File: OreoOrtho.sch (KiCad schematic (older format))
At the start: 31 parts, among them SW1 MXSwitch, SW2 MXSwitch, SW3 MXSwitch, SW4 MXSwitch, U1 ATmega32U2-AU, U2 PRTR5V0U2X, Y1 16MHz

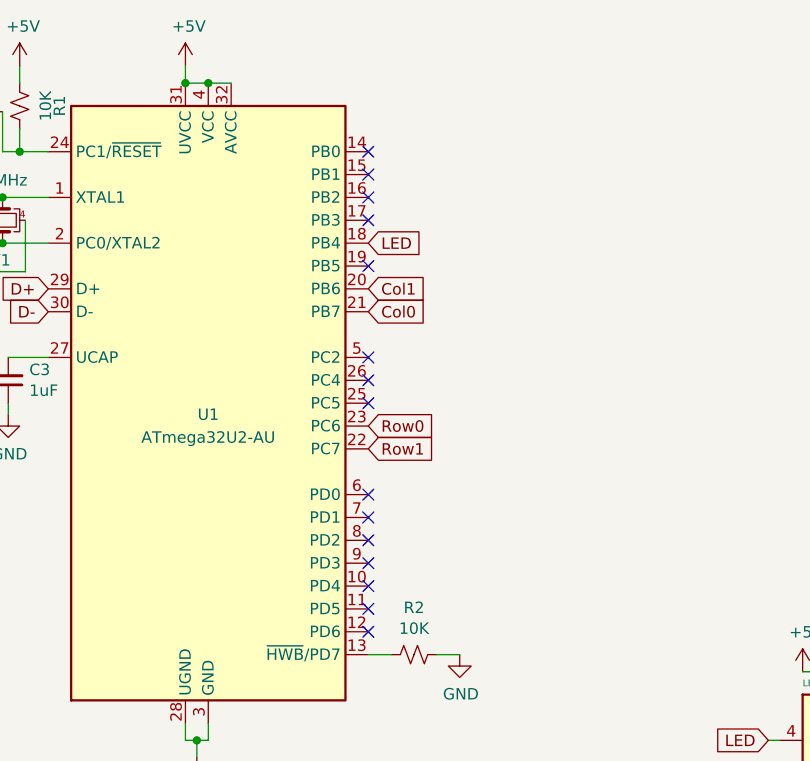
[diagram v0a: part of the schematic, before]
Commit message: reroute
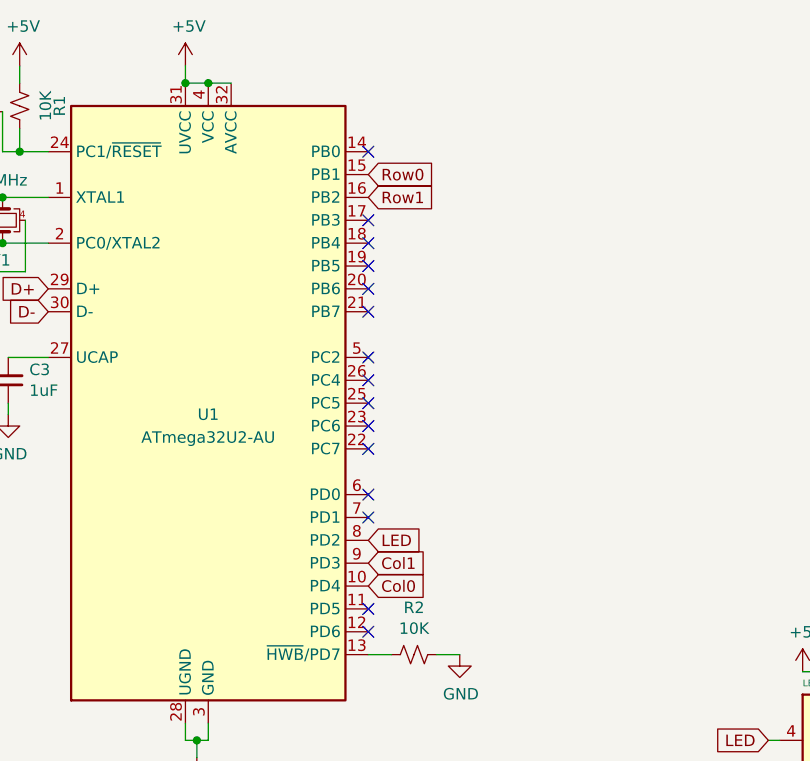
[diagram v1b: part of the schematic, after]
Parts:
- SW1, SW2, SW3, SW4: footprint kbd:CherryMX_1u -> kbd:CherryMX_Hotswap
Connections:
- net Col0: now also U1.10 (PD4); no longer U1.21 (PB7)
- net Col1: now also U1.9 (PD3); no longer U1.20 (PB6)
- net LED: now also U1.8 (PD2); no longer U1.18 (PB4)
- net Row0: now also U1.15 (PB1); no longer U1.23 (PC6)
- net Row1: now also U1.16 (PB2); no longer U1.22 (PC7)
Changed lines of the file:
@@
 Wire Wire Line
 	1925 4250 1925 4450
-Text GLabel 5825 2725 2    50   Input ~ 0
+Text GLabel 5825 1625 2    50   Input ~ 0
 Row1
-Text GLabel 5825 2025 2    50   Input ~ 0
+Text GLabel 5825 3225 2    50   Input ~ 0
 Col1
 $Comp
@@
 $EndComp
 NoConn ~ 5825 1425
-NoConn ~ 5825 1525
-NoConn ~ 5825 1625
+NoConn ~ 5825 2725
+NoConn ~ 5825 2625
 NoConn ~ 5825 2925
 NoConn ~ 5825 3025
-NoConn ~ 5825 3125
-NoConn ~ 5825 3225
-NoConn ~ 5825 3325
+NoConn ~ 5825 2025
+NoConn ~ 5825 1825
+NoConn ~ 5825 2125
 NoConn ~ 5825 3425
 NoConn ~ 5825 3525
@@
 F 0 "SW3" H 8250 1950 50  0000 L CNN
 F 1 "MXSwitch" H 8175 1875 39  0000 L CNN
-F 2 "kbd:CherryMX_1u" H 8325 1950 50  0001 C CNN
+F 2 "kbd:CherryMX_Hotswap" H 8325 1950 50  0001 C CNN
 F 3 "" H 8325 1950 50  0001 C CNN
 	1    8325 1950
@@
 F 0 "SW4" H 8950 1950 50  0000 L CNN
 F 1 "MXSwitch" H 8875 1875 39  0000 L CNN
-F 2 "kbd:CherryMX_1u" H 9025 1950 50  0001 C CNN
+F 2 "kbd:CherryMX_Hotswap" H 9025 1950 50  0001 C CNN
 F 3 "" H 9025 1950 50  0001 C CNN
 	1    9025 1950
@@
 F 0 "SW1" H 8250 1375 50  0000 L CNN
 F 1 "MXSwitch" H 8175 1300 39  0000 L CNN
-F 2 "kbd:CherryMX_1u" H 8325 1375 50  0001 C CNN
+F 2 "kbd:CherryMX_Hotswap" H 8325 1375 50  0001 C CNN
 F 3 "" H 8325 1375 50  0001 C CNN
 	1    8325 1375
@@
 	1    0    0    -1
 $EndComp
-Text GLabel 5825 2125 2    50   Input ~ 0
+Text GLabel 5825 3325 2    50   Input ~ 0
 Col0
-Text GLabel 5825 2625 2    50   Input ~ 0
+Text GLabel 5825 1525 2    50   Input ~ 0
 Row0
 NoConn ~ 5825 1725
-Text GLabel 5825 1825 2    50   Input ~ 0
+Text GLabel 5825 3125 2    50   Input ~ 0
 LED
 $Comp
@@
 F 0 "SW2" H 8950 1375 50  0000 L CNN
 F 1 "MXSwitch" H 8875 1300 39  0000 L CNN
-F 2 "kbd:CherryMX_1u" H 9025 1375 50  0001 C CNN
+F 2 "kbd:CherryMX_Hotswap" H 9025 1375 50  0001 C CNN
 F 3 "" H 9025 1375 50  0001 C CNN
 	1    9025 1375

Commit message: minor file changes
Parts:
- added C7: 0.1uF, Capacitor_SMD:C_0603_1608Metric, symbol Device:C_Small
- added G2: Oreo, doggy:bike, symbol oreo:LOGO
- SW1, SW2, SW3, SW4: footprint kbd:CherryMX_Hotswap -> doggy:CherryMX_Hotswap_clear
- U1: value ATmega32U2-AU -> ATmega32U4-AU; footprint Package_QFP:TQFP-32_7x7mm_P0.8mm -> Package_QFP:TQFP-44_10x10mm_P0.8mm; symbol MCU_Microchip_ATmega:ATmega32U2-AU -> MCU_Microchip_ATmega:ATmega32U4-AU
- USB1: footprint Type-C:HRO-TYPE-C-31-M-12-Assembly -> Type-C:HRO-TYPE-C-31-M-12
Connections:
- net +5V: now also U1.14 (VCC), U1.2 (UVCC), U1.24 (AVCC), U1.34 (VCC), U1.44 (AVCC), U1.7 (VBUS), C7.2; no longer U1.31 (UVCC), U1.32 (AVCC), U1.4 (VCC)
- net Col0: now also U1.12 (PB7); no longer U1.10 (PD4)
- net Col1: now also U1.11 (PB3); no longer U1.9 (PD3)
- net D+: now also U1.4 (D+); no longer U1.29 (D+)
- net D-: now also U1.3 (D-); no longer U1.30 (D-)
- net GND: now also U1.15 (GND), U1.23 (GND), U1.35 (GND), U1.43 (GND), U1.5 (UGND), C7.1; no longer U1.28 (UGND), U1.3 (GND)
- net Row0: now also U1.29 (PB5); no longer U1.15 (PB1)
- net Row1: now also U1.30 (PB6); no longer U1.16 (PB2)
- net at C3.2: now also U1.6 (UCAP); no longer U1.27 (UCAP)
- net at R2.2: now also U1.33 (~HWB~/PE2); no longer U1.13 (~HWB~/PD7)
- net at C1.2, Y1.1: now also U1.17 (XTAL1); no longer U1.1 (XTAL1)
- net at C2.2, Y1.3: now also U1.16 (XTAL2); no longer U1.2 (PC0/XTAL2)
- net RST: now reaches R1.1, RST_SW1.2
- net RST: now also U1.13 (~RESET); no longer U1.24 (PC1/~RESET)
- no-connect marks 18 -> 24
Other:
- moved on the sheet: C1, C2, C3, C4, C5, C6, D1, D2, D3, D4, F1, H1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
